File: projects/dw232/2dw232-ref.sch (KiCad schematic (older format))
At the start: 29 parts, among them Q501 MMBT3904, Q502 MMBT3904, U501 LM741, U502 LM741, U503 2DW232

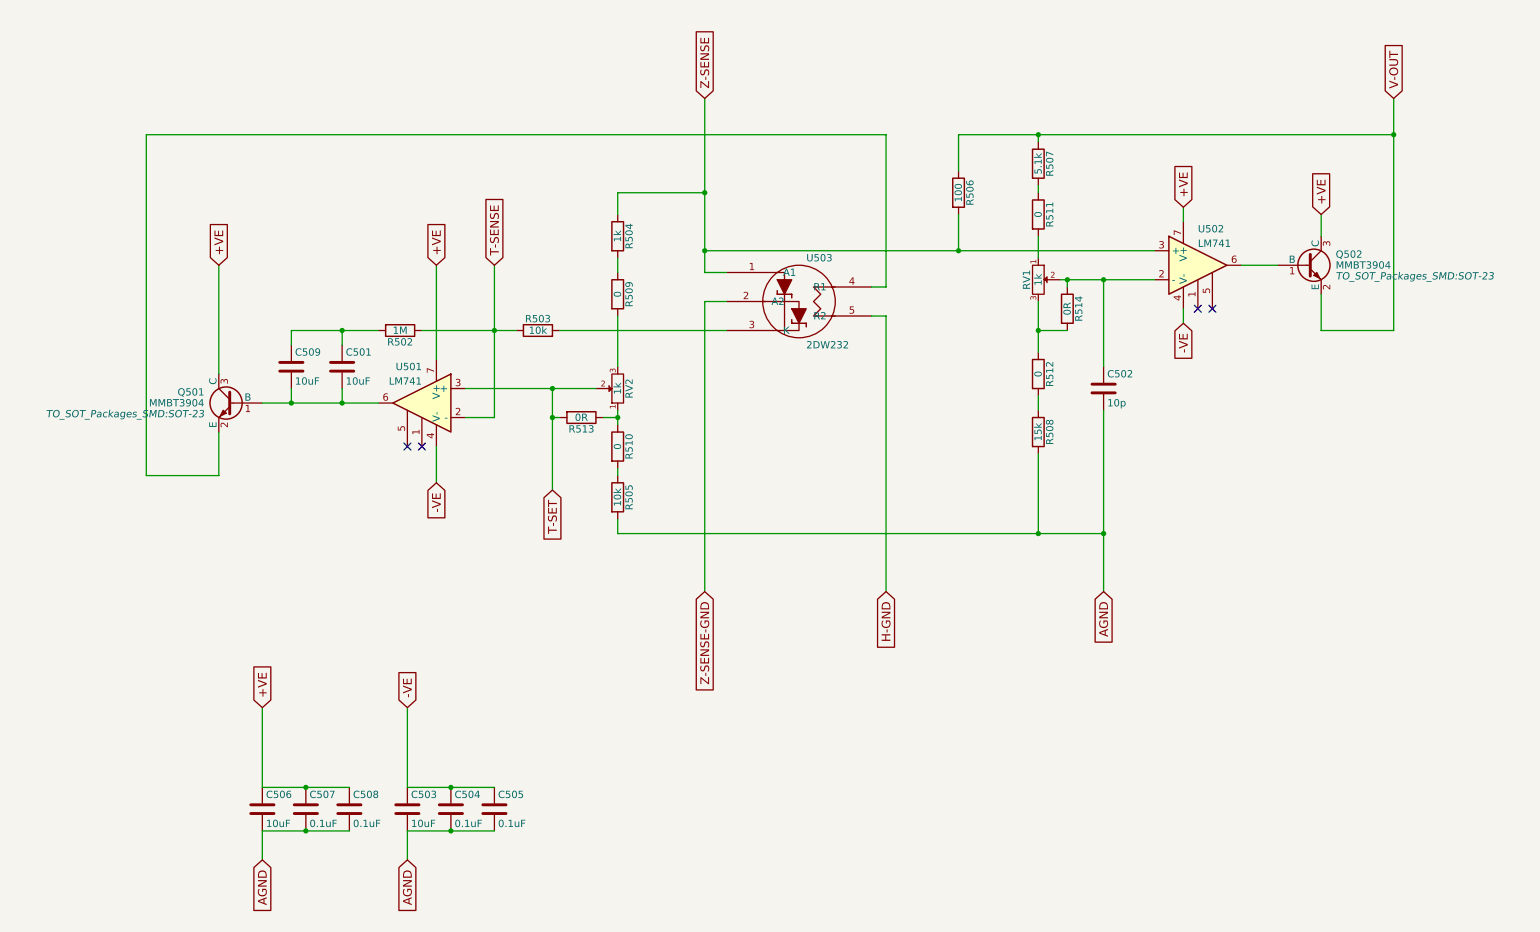
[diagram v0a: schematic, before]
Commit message: fix schematic v0.3
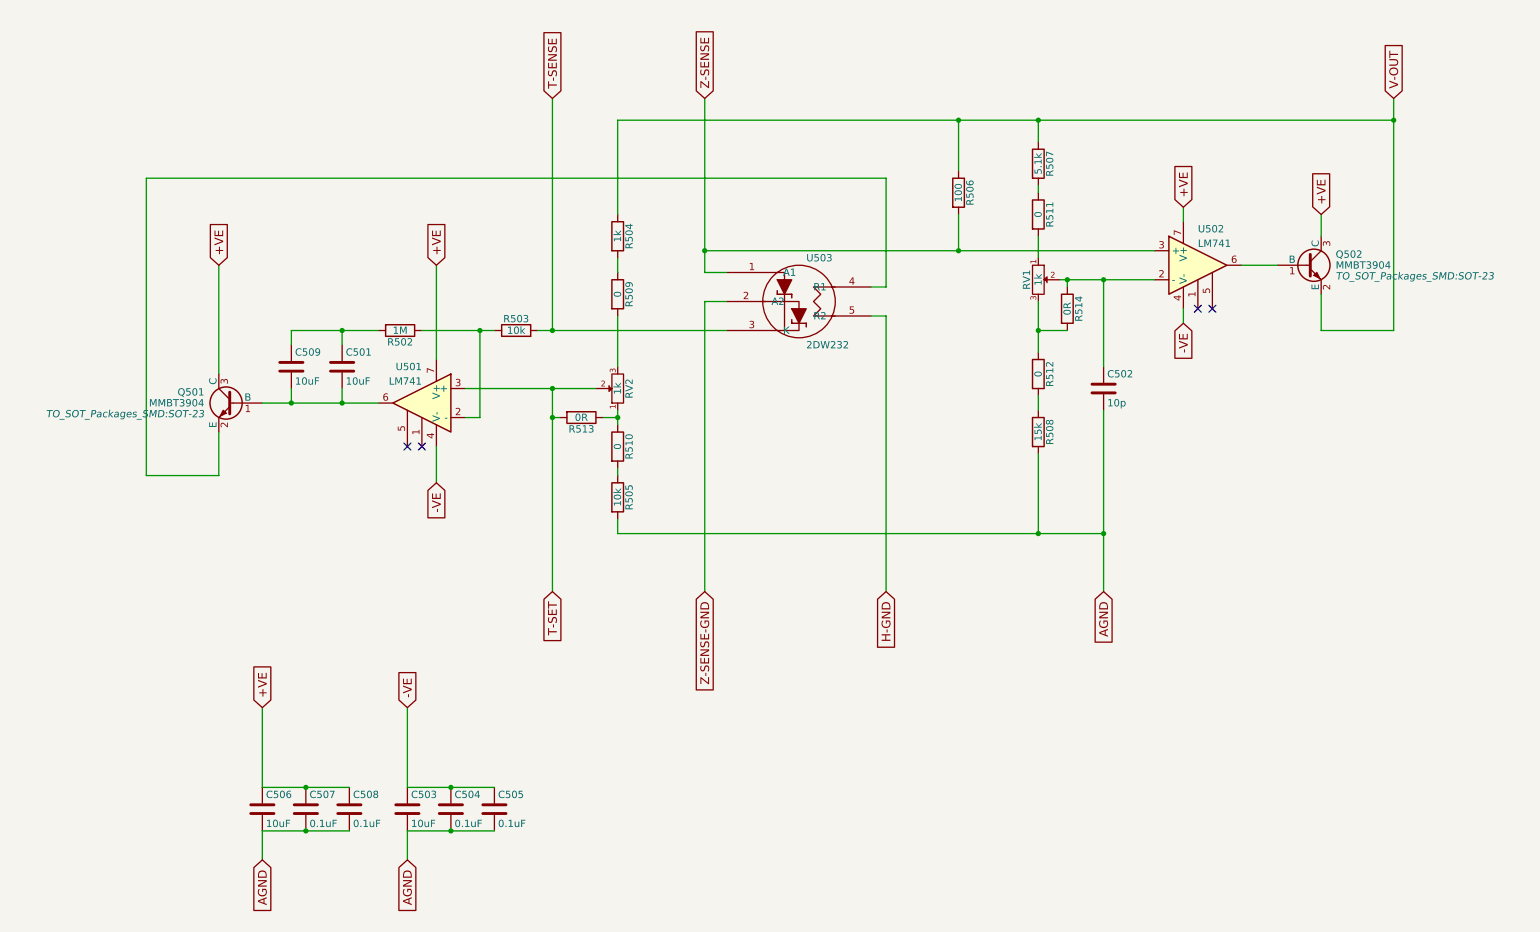
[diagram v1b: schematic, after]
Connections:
- net T-SENSE: now also R503.2, U503.3 (K); no longer R502.1, R503.1, U501.2 (-)
- net V-OUT: now also R504.1
- net Z-SENSE: no longer R504.1
- new net: R502.1, R503.1, U501.2 (-)
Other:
- moved on the sheet: R503
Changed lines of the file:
@@
 L R R503
 U 1 1 5881B3DC
-P 3600 2700
-F 0 "R503" V 3680 2700 50  0000 C CNN
-F 1 "10k" V 3600 2700 50  0000 C CNN
-F 2 "Resistors_SMD:R_1206" V 3530 2700 50  0001 C CNN
-F 3 "" H 3600 2700 50  0000 C CNN
-	1    3600 2700
+P 3450 2700
+F 0 "R503" V 3530 2700 50  0000 C CNN
+F 1 "10k" V 3450 2700 50  0000 C CNN
+F 2 "Resistors_SMD:R_1206" V 3380 2700 50  0001 C CNN
+F 3 "" H 3450 2700 50  0000 C CNN
+	1    3450 2700
 	0    -1   -1   0
 $EndComp
@@
 	1    0    0    -1
 $EndComp
-Text GLabel 3300 2250 1    60   Input ~ 0
+Text GLabel 3700 1100 1    60   Input ~ 0
 T-SENSE
-Text GLabel 3700 3800 3    60   Input ~ 0
+Text GLabel 3700 4500 3    60   Input ~ 0
 T-SET
 Text GLabel 9500 1100 1    60   Input ~ 0
@@
 	7050 1700 7050 1750
 Wire Wire Line
-	3100 3100 4000 3100
+	3100 3100 3700 3100
+Wire Wire Line
+	3700 3100 4000 3100
 Wire Wire Line
 	4150 3650 4150 3650
@@
 Connection ~ 2000 5850
 Wire Wire Line
-	1700 6150 2300 6150
-Wire Wire Line
-	1700 5850 2300 5850
+	1700 6150 2000 6150
+Wire Wire Line
+	2000 6150 2300 6150
+Wire Wire Line
+	1700 5850 2000 5850
+Wire Wire Line
+	2000 5850 2300 5850
 Wire Wire Line
 	1700 5300 1700 5850
@@
 Connection ~ 4750 2150
 Wire Wire Line
-	6500 1350 6500 1600
-Wire Wire Line
-	4750 1100 4750 2300
+	6500 1250 6500 1600
+Wire Wire Line
+	4750 1100 4750 2150
+Wire Wire Line
+	4750 2150 4750 2300
 Wire Wire Line
 	4750 2300 4900 2300
 Wire Wire Line
-	3750 2700 4900 2700
+	3600 2700 3700 2700
+Wire Wire Line
+	3700 2700 4900 2700
 Wire Wire Line
 	4750 2500 4750 4500
@@
 Connection ~ 3000 5850
 Wire Wire Line
-	2700 6150 3300 6150
-Wire Wire Line
-	2700 5850 3300 5850
+	2700 6150 3000 6150
+Wire Wire Line
+	3000 6150 3300 6150
+Wire Wire Line
+	2700 5850 3000 5850
+Wire Wire Line
+	3000 5850 3300 5850
 Wire Wire Line
 	7050 3150 7050 3250
 Connection ~ 7500 4100
 Wire Wire Line
-	7500 3250 7500 4500
-Wire Wire Line
-	4150 4100 7500 4100
+	7500 3250 7500 4100
+Wire Wire Line
+	7500 4100 7500 4500
+Wire Wire Line
+	4150 4100 7050 4100
+Wire Wire Line
+	7050 4100 7500 4100
 Wire Wire Line
 	7050 4100 7050 3550
@@
 	9500 2700 9000 2700
 Wire Wire Line
-	9500 1100 9500 2700
+	9500 1100 9500 1250
+Wire Wire Line
+	9500 1250 9500 2700
 Wire Wire Line
 	1400 2250 1400 3000
@@
 	2900 2250 2900 2900
 Wire Wire Line
-	1700 3200 2500 3200
+	1700 3200 1900 3200
+Wire Wire Line
+	1900 3200 2250 3200
+Wire Wire Line
+	2250 3200 2500 3200
 Wire Wire Line
 	2250 3200 2250 3100
@@
 	2250 2700 2250 2800
 Wire Wire Line
-	1900 2700 2500 2700
-Connection ~ 3300 2700
-Wire Wire Line
-	3300 3300 3100 3300
-Wire Wire Line
-	3300 2250 3300 3300
-Wire Wire Line
-	2800 2700 3450 2700
+	1900 2700 2250 2700
+Wire Wire Line
+	2250 2700 2500 2700
+Connection ~ 3200 2700
+Wire Wire Line
+	3200 3300 3100 3300
+Wire Wire Line
+	3200 2700 3200 3300
+Wire Wire Line
+	2800 2700 3200 2700
+Wire Wire Line
+	3200 2700 3300 2700
 Wire Wire Line
 	4150 2200 4150 2300
@@
 Wire Wire Line
 	7500 2350 7500 2950
-Connection ~ 7050 1350
+Connection ~ 7050 1250
 Connection ~ 7050 4100
 Wire Wire Line
 	8050 1850 8050 1950
 Wire Wire Line
-	7050 1350 7050 1400
+	7050 1250 7050 1400
 Wire Wire Line
 	2700 5300 2700 5850
 Wire Wire Line
-	7050 2500 7050 2850
+	7050 2500 7050 2700
+Wire Wire Line
+	7050 2700 7050 2850
 Wire Wire Line
 	7050 2050 7050 2200
@@
 Connection ~ 7250 2350
 Wire Wire Line
-	4150 3250 4150 3350
+	4150 3250 4150 3300
+Wire Wire Line
+	4150 3300 4150 3350
 Wire Wire Line
 	4150 2600 4150 2950
@@
 	3750 3300 3700 3300
 Wire Wire Line
-	3700 3100 3700 3800
+	3700 3100 3700 3300
+Wire Wire Line
+	3700 3300 3700 4500
 Connection ~ 3700 3100
 Connection ~ 3700 3300
@@
 Connection ~ 6500 2150
 Wire Wire Line
-	4750 2150 7850 2150
+	4750 2150 6500 2150
+Wire Wire Line
+	6500 2150 7850 2150
 Wire Wire Line
 	4150 4000 4150 4100
 Wire Wire Line
-	7200 2350 7850 2350
+	7200 2350 7250 2350
+Wire Wire Line
+	7250 2350 7500 2350
+Wire Wire Line
+	7500 2350 7850 2350
 Wire Wire Line
 	1400 3700 900  3700
 Wire Wire Line
-	900  3700 900  1350
-Wire Wire Line
-	900  1350 6000 1350
+	900  3700 900  1650
+Wire Wire Line
+	900  1650 6000 1650
 Wire Wire Line
 	1400 3700 1400 3400
 Wire Wire Line
-	6000 1350 6000 2400
-Wire Wire Line
-	4150 1750 4750 1750
-Connection ~ 4750 1750
-Wire Wire Line
-	4150 1750 4150 1900
-Connection ~ 9500 1350
-Wire Wire Line
-	6500 1350 9500 1350
+	4150 1250 4150 1900
+Connection ~ 9500 1250
+Wire Wire Line
+	4150 1250 6500 1250
+Wire Wire Line
+	6500 1250 7050 1250
+Wire Wire Line
+	7050 1250 9500 1250
+Wire Wire Line
+	6000 1650 6000 2400
+Connection ~ 6500 1250
+Wire Wire Line
+	3700 1100 3700 2700
+Connection ~ 3700 2700
 $EndSCHEMATC
